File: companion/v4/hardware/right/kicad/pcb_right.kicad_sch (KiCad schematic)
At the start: 40 parts, among them J1 TF31-6S-0.5SH_800_, J2 speaker, J3 USB_C_Receptacle_USB2.0_14P, J4 Conn_01x24_MountingPin, SW1 SW_Push, SW2 SW_Push, U1 AP2112K-3.3, U2 MAX98357AETE_T, U3 ESP32-C6-MINI-1, U4 ESP32-S3-MINI-1, U5 TLV75528PDBV, U7 TLV75515PDBV

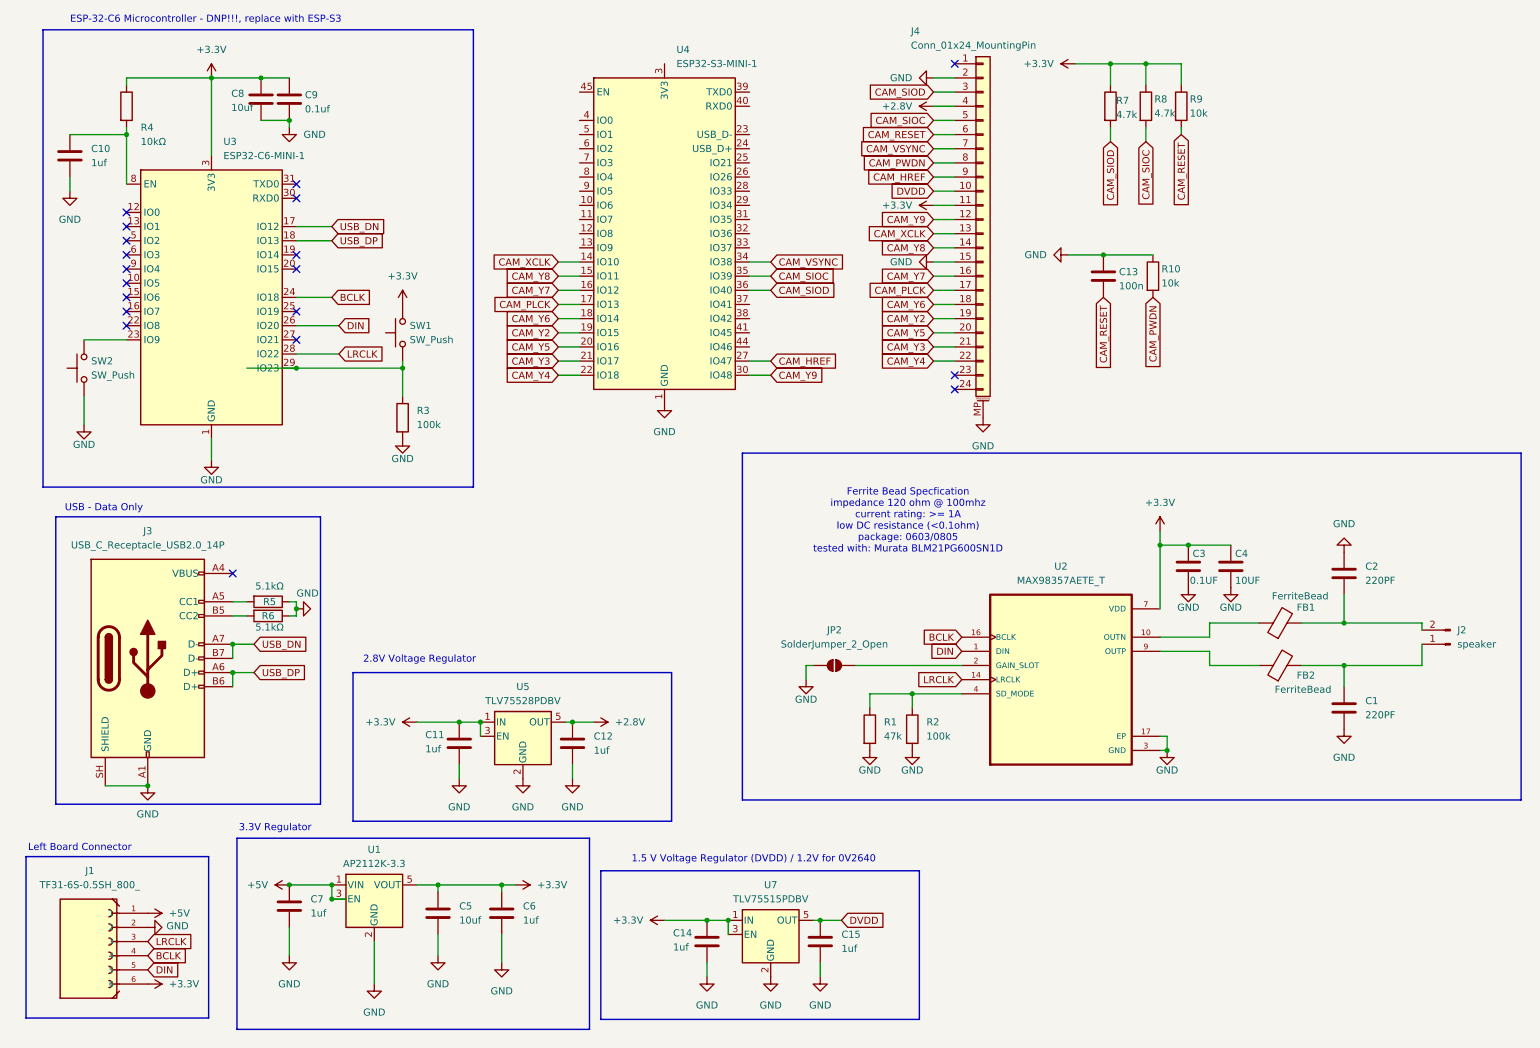
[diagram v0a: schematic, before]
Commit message: ESP-32-S3
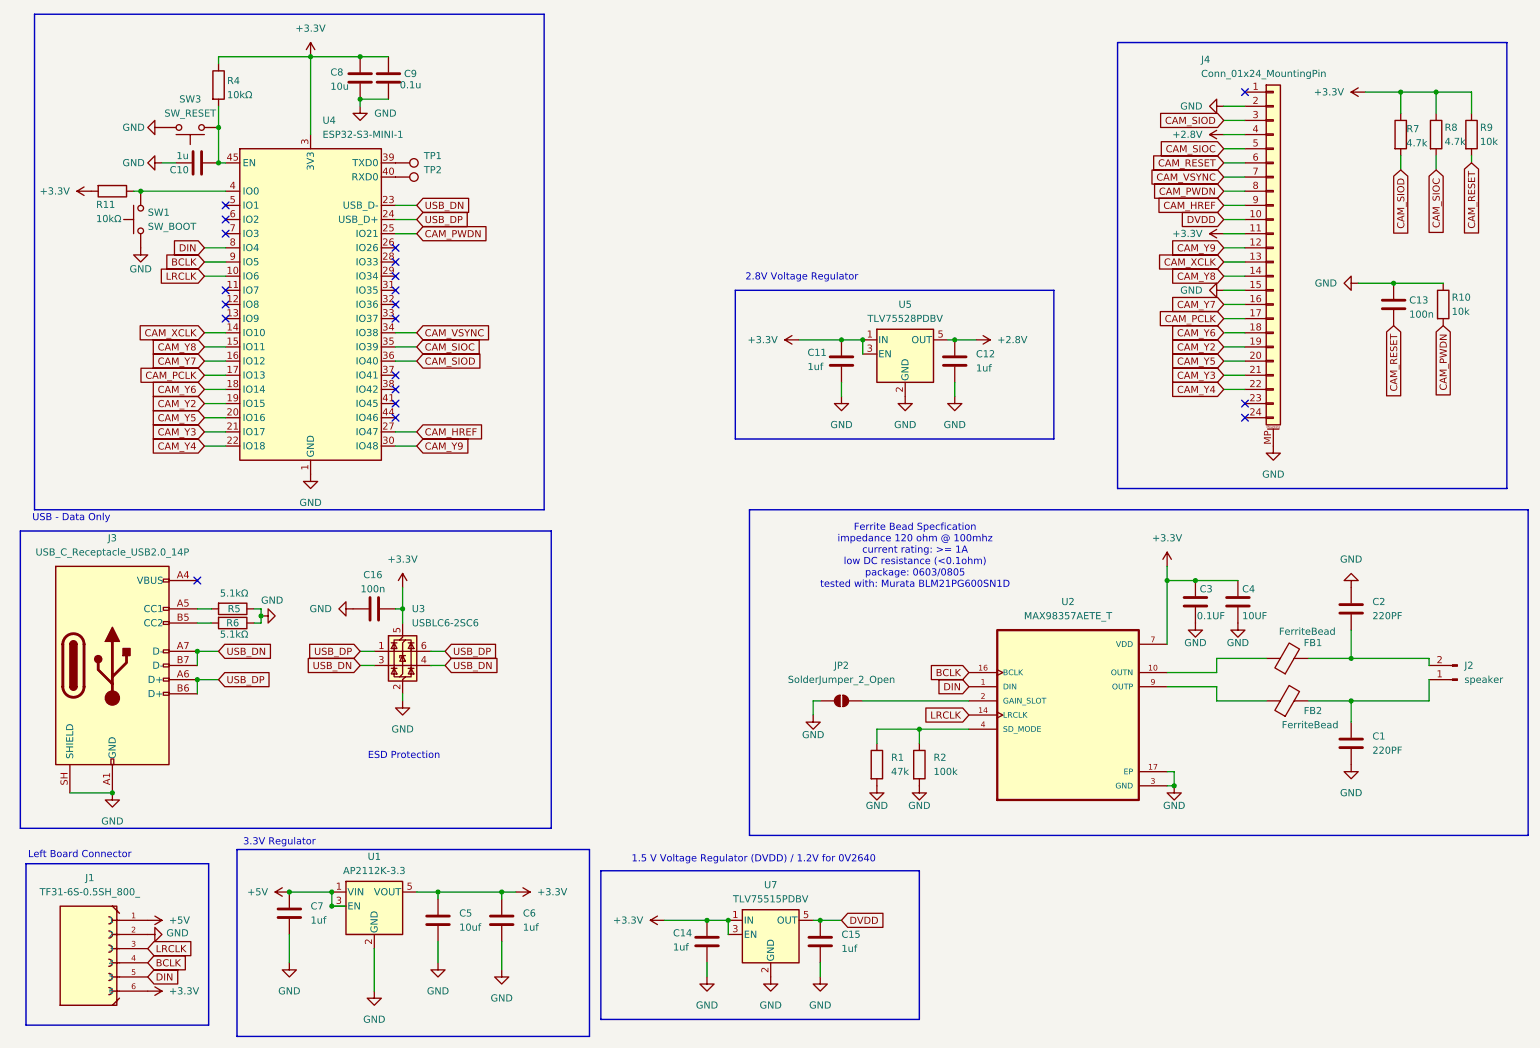
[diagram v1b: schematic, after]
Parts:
- removed R3: 100k, Resistor_SMD:R_0805_2012Metric_Pad1.20x1.40mm_HandSolder, symbol Device:R
- removed SW2: SW_Push, symbol Switch:SW_Push
- removed U3: ESP32-C6-MINI-1, RF_Module:ESP32-C6-MINI-1, symbol RF_Module:ESP32-C6-MINI-1
- added C16: 100n, symbol Device:C
- added R11: 10kΩ, symbol Device:R
- added SW3: SW_RESET, Button_Switch_THT:SW_PUSH_6mm_H5mm, symbol Switch:SW_Push
- added TP1: TestPoint, Package_TO_SOT_SMD:SOT-23-5, symbol Connector:TestPoint
- added TP2: TestPoint, symbol Connector:TestPoint
- added U3: USBLC6-2SC6, Package_TO_SOT_SMD:SOT-23-6, symbol Power_Protection:USBLC6-2SC6
- C10: value 1uf -> 1u
- C8: value 10uf -> 10u
- C9: value 0.1uf -> 0.1u
- SW1: value SW_Push -> SW_BOOT
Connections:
- net +3.3V: now also U4.3 (3V3), C16.2, R11.2, U3.5 (VBUS); no longer SW1.2
- net BCLK: now also U4.9 (IO5)
- net CAM_PWDN: now also U4.25 (IO21)
- net DIN: now also U4.8 (IO4)
- net GND: now also SW1.1, C16.1, SW3.2, U3.2 (GND)
- net LRCLK: now also U4.10 (IO6)
- net USB_DN: now also U4.23 (USB_D-), U3.3 (I/O2), U3.4 (I/O2)
- net USB_DP: now also U4.24 (USB_D+), U3.1 (I/O1), U3.6 (I/O1)
- net at C10.1, R4.2: now also U4.45 (EN), SW3.1
- net at U4.39 (TXD0): now also TP1.1
- net at U4.4 (IO0): now also SW1.2, R11.1
- net at U4.40 (RXD0): now also TP2.1
- net CAM_PLCK renamed CAM_PCLK
- no-connect marks 19 -> 20
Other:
- note added: "ESD Protection"
- note removed: "ESP-32-C6 Microcontroller - DNP!!!, replace with ESP-S3"
- moved on the sheet: C1, C11, C12, C13, C2, C3, C4, C5, C6, C7, FB1, FB2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
